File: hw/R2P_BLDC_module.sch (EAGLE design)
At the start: 68 parts, among them Q1 OPTIMOS, Q2 OPTIMOS, Q3 OPTIMOS, Q4 OPTIMOS, Q5 OPTIMOS, Q6 OPTIMOS, U1 STM32F103CX, X1 MICROMATCH-4

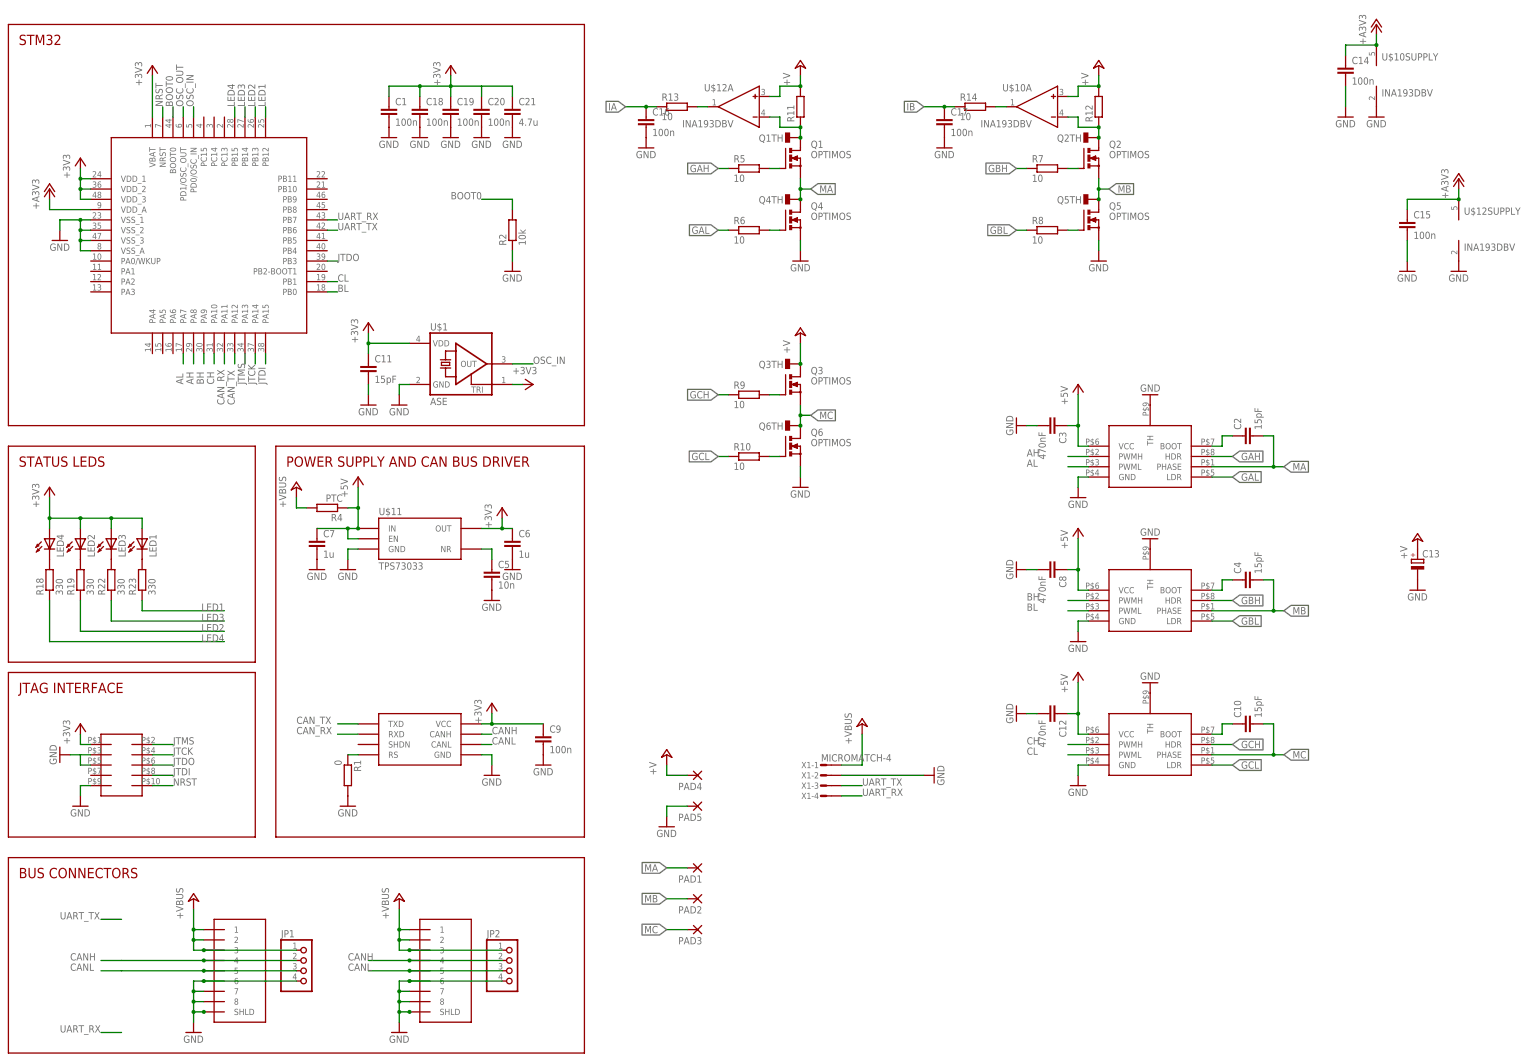
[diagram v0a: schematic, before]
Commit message: started layout
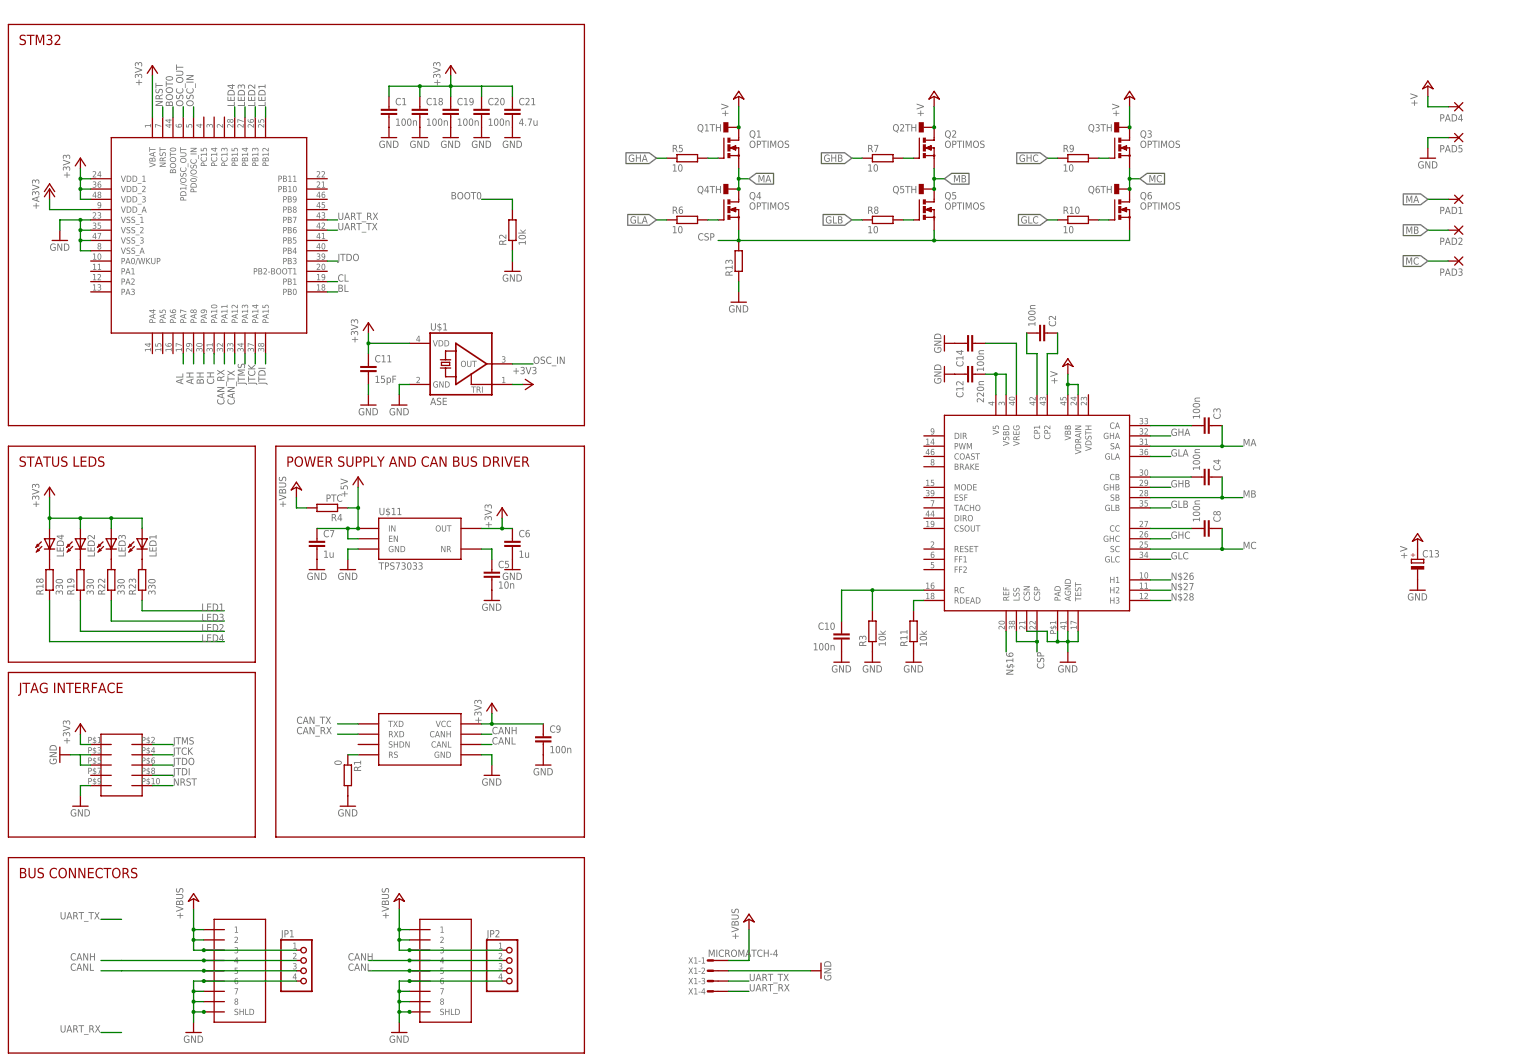
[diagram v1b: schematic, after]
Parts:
- removed C15, C16, C17: 100n, rcl:C-EUC0603
- removed R12: (no value), rcl:R-EU_R1206
- removed R14: 10, rcl:R-EU_R0603
- removed U$10, U$12: INA193DBV, texas-instruments:INA193DBV
- removed U$8, U$9: MCP14700MF, microchip:MCP14700MF
- added R3: 10k, rcl:R-EU_R0603
- C10, C2, C4: value 15pF -> 100n
- C12: value 470nF -> 220n
- C3, C8: value 470nF -> 100n
- R11: value (none) -> 10k; device rcl:R-EU_R1206 -> rcl:R-EU_R0603
- R13: value 10 -> (none); device rcl:R-EU_R0603 -> rcl:R-EU_R2512
- U$2: value MCP14700MF -> A3930; device microchip:MCP14700MF -> allegro:A3930
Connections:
- removed net GAH: R5.1, U$2.HDR
- removed net GAL: R6.1, U$2.LDR
- removed net GBH: R7.1, U$8.HDR
- removed net GBL: R8.1, U$8.LDR
- removed net GCH: R9.1, U$9.HDR
- removed net GCL: R10.1, U$9.LDR
- removed net IA: C16.1, R13.1
- removed net IB: C17.1, R14.1
- new net CSP: Q4G$1.S, Q5G$1.S, Q6G$1.S, R13.2, U$2.CSP, U$2.LSS
- new net GHA: R5.1, U$2.GHA
- new net GHB: R7.1, U$2.GHB
- new net GHC: R9.1, U$2.GHC
- new net GLA: R6.1, U$2.GLA
- new net GLB: R8.1, U$2.GLB
- new net GLC: R10.1, U$2.GLC
- new net N$21: C12.2, U$2.V5, U$2.V5BD
- new net N$23: C14.2, U$2.VREG
- new net N$26: U$2.H1
- new net N$27: U$2.H2
- new net N$28: U$2.H3
- new net N$3: C3.2, U$2.CA
- net +5V: no longer C12.1, C3.1, C8.1, U$2.VCC, U$8.VCC, U$9.VCC
- net +A3V3: no longer C14.1, C15.1, U$10SUPPLY.V+, U$12SUPPLY.V+
- net +V: now also Q1G$1.D, Q1TH.TH, Q2G$1.D, Q2TH.TH, U$2.VBB, U$2.VDRAIN; no longer R11.2, R12.2, U$10A.IN+, U$12A.IN+
- net AH: no longer U$2.PWMH
- net AL: no longer U$2.PWML
- net BH: no longer U$8.PWMH
- net BL: no longer U$8.PWML
- net CH: no longer U$9.PWMH
- net CL: no longer U$9.PWML
- net GND: now also C10.2, C12.1, C14.1, R11.1, R13.1, R3.1, U$2.AGND, U$2.CSN, U$2.PAD, U$2.TEST; no longer C12.2, C14.2, C15.2, C16.2, C17.2, C3.2, C8.2, Q4G$1.S, Q5G$1.S, Q6G$1.S, U$10SUPPLY.V-, U$12SUPPLY.V-, U$2.GND, U$2.TH, U$8.GND, U$8.TH, U$9.GND, U$9.TH
- net MA: now also C3.1, U$2.SA; no longer C2.2, U$2.PHASE
- net MB: now also C4.1, U$2.SB; no longer C4.2, U$8.PHASE
- net MC: now also C8.1, U$2.SC; no longer C10.2, U$9.PHASE
- net N$10: now also C2.1, U$2.CP2; no longer C10.1, U$9.BOOT
- net N$14: now also C4.2, U$2.CB; no longer Q1G$1.D, Q1TH.TH, R11.1, U$12A.IN-
- net N$16: now also U$2.REF; no longer Q2G$1.D, Q2TH.TH, R12.1, U$10A.IN-
- net N$17: now also C10.1, R3.2, U$2.RC; no longer R13.2, U$12A.OUT
- net N$19: now also C8.2, U$2.CC; no longer R14.2, U$10A.OUT
- net N$5: now also C2.2, U$2.CP1; no longer C4.1, U$8.BOOT
- net N$6: now also R11.2, U$2.RDEAD; no longer C2.1, U$2.BOOT
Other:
- moved on the sheet: C10, C12, C14, C2, C3, C4, C8, PAD1, PAD2, PAD3, PAD4, PAD5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
